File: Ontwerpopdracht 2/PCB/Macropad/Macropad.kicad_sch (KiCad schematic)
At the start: 15 parts, among them IC1 PEC12R-4220F-S0024, IC2 PEC12R-4220F-S0024

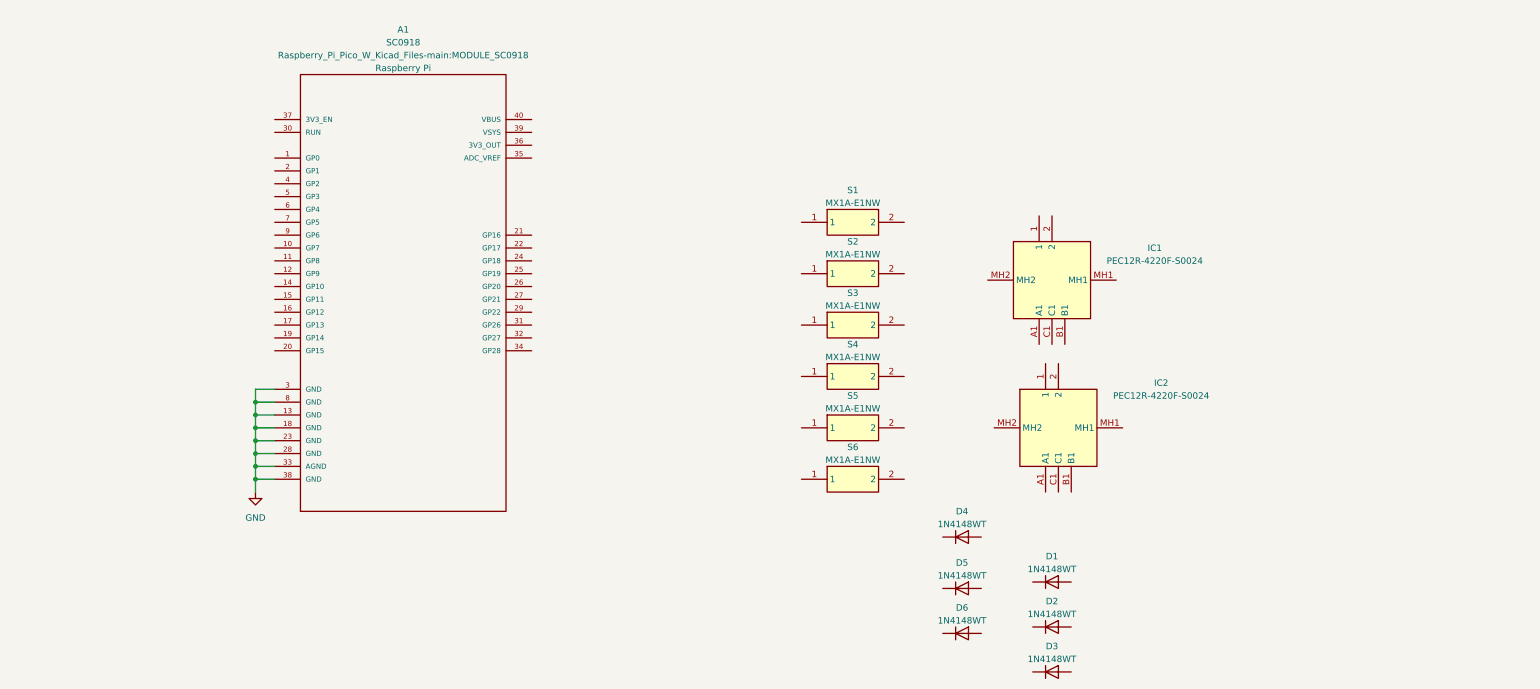
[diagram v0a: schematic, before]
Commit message: pcb
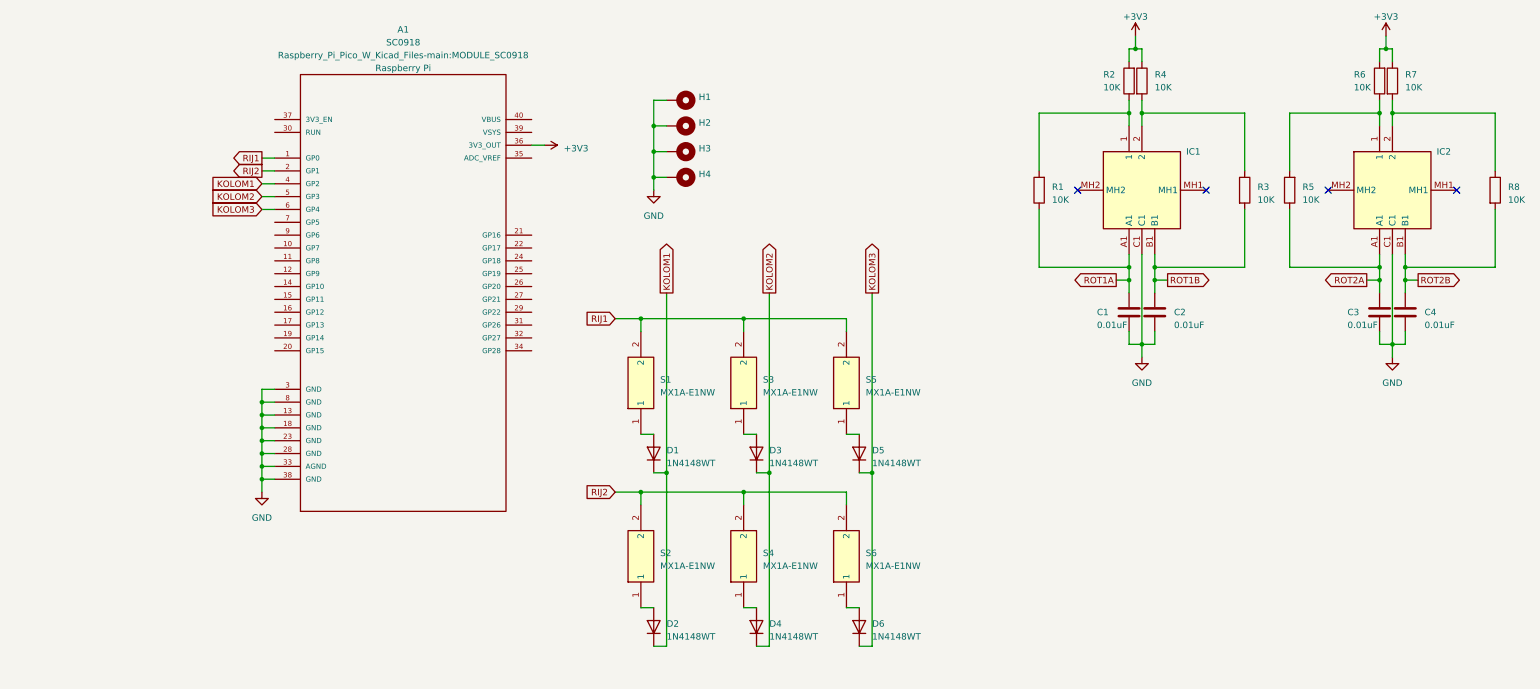
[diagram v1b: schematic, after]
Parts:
- added C1, C2, C3, C4: 0.01uF, Capacitor_SMD:C_0805_2012Metric_Pad1.18x1.45mm_HandSolder, symbol Device:C
- added H1, H2, H3, H4: MountingHole_Pad, MountingHole:MountingHole_2.2mm_M2_Pad_Via, symbol Mechanical:MountingHole_Pad
- added R1, R2, R3, R4, R5, R6, R7, R8: 10K, Resistor_SMD:R_0805_2012Metric_Pad1.20x1.40mm_HandSolder, symbol Device:R
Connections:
- net GND: now also IC1.C1, IC2.C1, C1.2, C2.2, C3.2, C4.2, H1.1, H2.1, H3.1, H4.1
- net at S6.1: now also D6.2 (A)
- net RIJ2: now reaches S6.2
- net RIJ2: now also A1.2 (GP1), S2.2, S4.2
- net KOLOM3: now reaches D5.1 (K)
- net KOLOM3: now also A1.6 (GP4), D6.1 (K)
- net at D5.2 (A): now also S5.1
- net at S2.1: now also D2.2 (A)
- net RIJ1: now reaches A1.1 (GP0)
- net RIJ1: now also S1.2, S3.2, S5.2
- net +3V3: now reaches A1.36 (3V3_OUT)
- net +3V3: now also R2.2, R4.1, R6.2, R7.1
- net KOLOM1: now reaches A1.4 (GP2)
- net KOLOM1: now also D1.1 (K), D2.1 (K)
- net KOLOM2: now reaches A1.5 (GP3)
- net KOLOM2: now also D3.1 (K), D4.1 (K)
- net at D4.2 (A): now also S4.1
- net at D1.2 (A): now also S1.1
- net at IC1.1: now also R1.2, R2.1
- net at IC1.2: now also R3.1, R4.2
- net ROT1A: now reaches IC1.A1
- net ROT1A: now also C1.1, R1.1
- net ROT1B: now reaches IC1.B1
- net ROT1B: now also C2.1, R3.2
- net at S3.1: now also D3.2 (A)
- net at IC2.1: now also R5.2, R6.1
- net at IC2.2: now also R7.2, R8.1
- net ROT2A: now reaches IC2.A1
- net ROT2A: now also C3.1, R5.1
- net ROT2B: now reaches IC2.B1
- net ROT2B: now also C4.1, R8.2
- no-connect marks 0 -> 4
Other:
- moved on the sheet: D1, D2, D3, D4, D5, D6, IC1, S1, S2, S3, S4, S5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

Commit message: pcb klaar
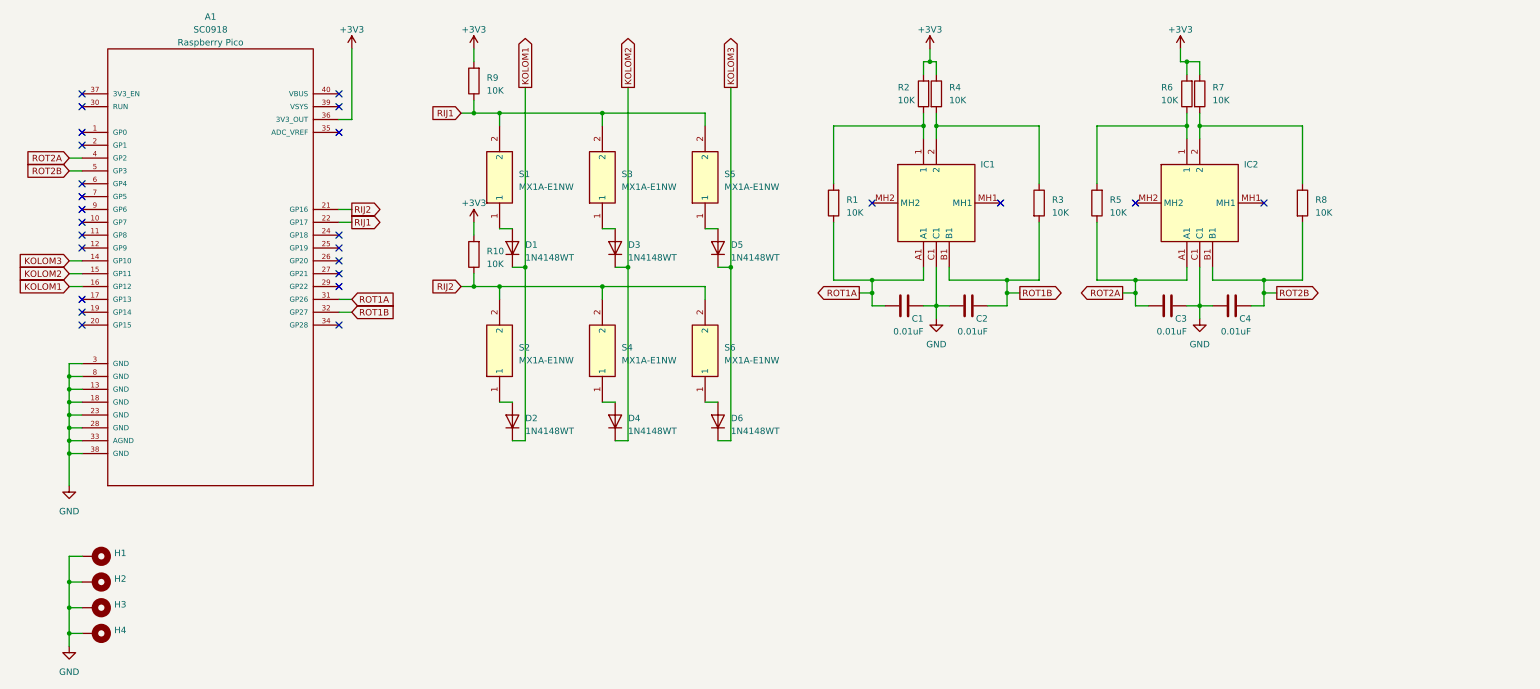
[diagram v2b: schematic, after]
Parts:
- added R10, R9: 10K, Resistor_SMD:R_0805_2012Metric_Pad1.20x1.40mm_HandSolder, symbol Device:R
- A1: manufacturer Raspberry Pi -> Raspberry Pico
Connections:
- net +3V3: now also R10.2, R9.2
- net GND: now also C2.1, C4.1; no longer C2.2, C4.2
- net KOLOM1: now also A1.16 (GP12); no longer A1.4 (GP2)
- net KOLOM2: now also A1.15 (GP11); no longer A1.5 (GP3)
- net KOLOM3: now also A1.14 (GP10); no longer A1.6 (GP4)
- net RIJ1: now also A1.22 (GP17), R9.1; no longer A1.1 (GP0)
- net RIJ2: now also A1.21 (GP16), R10.1; no longer A1.2 (GP1)
- net ROT1A: now also A1.31 (GP26)
- net ROT1B: now also A1.32 (GP27), C2.2; no longer C2.1
- net ROT2A: now also A1.4 (GP2)
- net ROT2B: now also A1.5 (GP3), C4.2; no longer C4.1
- no-connect marks 4 -> 26
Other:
- moved on the sheet: A1, C1, C2, C3, C4, D1, D2, D3, D4, D5, D6, H1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
